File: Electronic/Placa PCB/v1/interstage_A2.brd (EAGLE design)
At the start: 82.5 x 29 mm, 22 parts, among them J1 0532611271, J2 0532611271, Q1 PMV16XNR, U2 ATMEGA328P_TQFP, Y1 16MHz

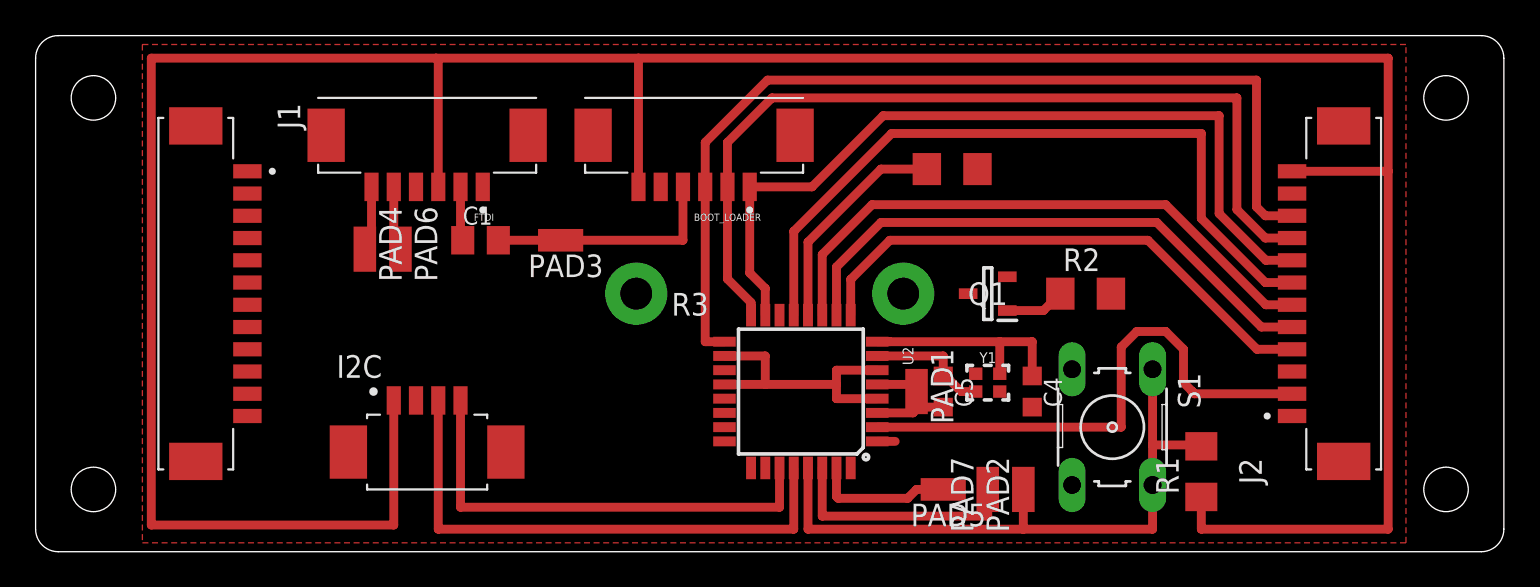
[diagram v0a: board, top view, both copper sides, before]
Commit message: Avance
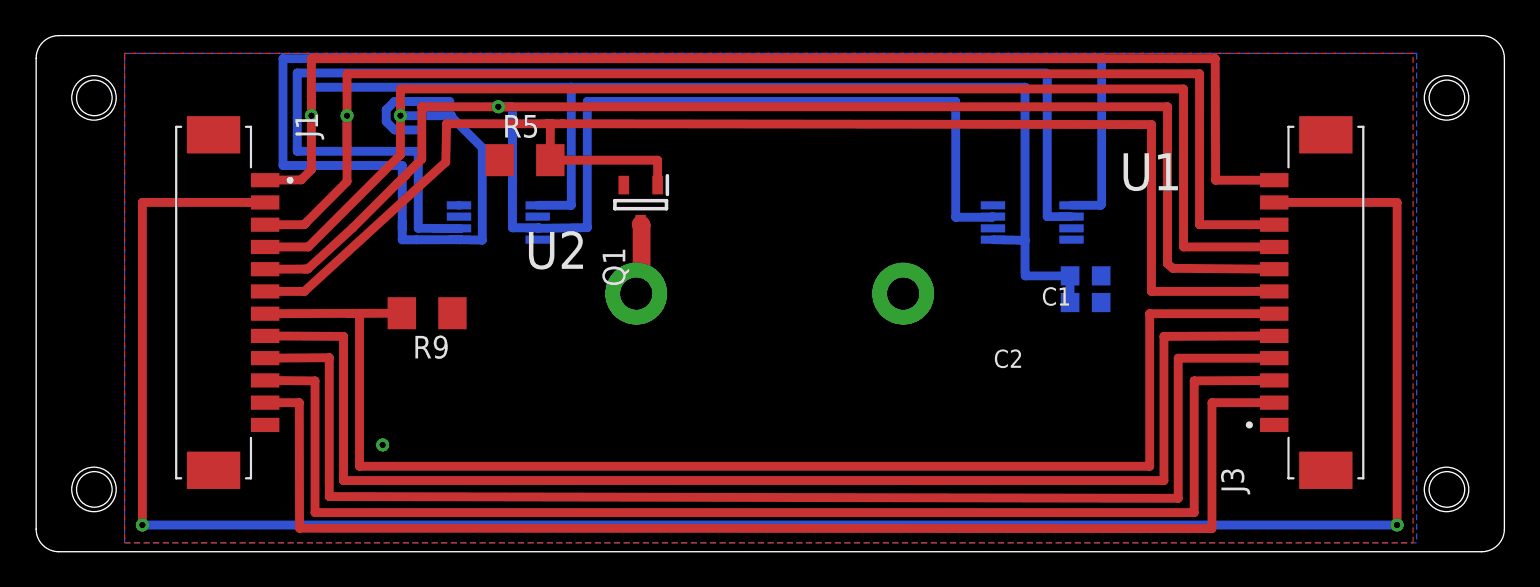
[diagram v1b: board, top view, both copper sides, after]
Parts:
- removed BOOT_LOADER, FTDI: 0532610671, picoblade6:MOLEX_0532610671
- removed C4, C5: 22pF, rcl:C0603K
- removed I2C: 0532610471, 0532610471:MOLEX_0532610471
- removed J2: 0532611271, picoblade:MOLEX_0532611271
- removed PAD1, PAD2, PAD3, PAD4, PAD5, PAD6, PAD7: WIREPADSMD1,27-254, wirepad:SMD1,27-2,54
- removed R1: 10kohm, rcl:R1206
- removed R2, R3: 330 Ohm, rcl:R1206
- removed S1: (no value), switch-omron:B3F-10XX
- removed Y1: 16MHz, SparkFun-Clocks:CRYSTAL-SMD-2.0X1.6MM
- added C2: 0.1pF, rcl:C0603K
- added J3: 0532611271, picoblade:MOLEX_0532611271
- added R5, R9: 330 Ohm, rcl:R1206
- added U1: LM70CIMM-3, LM70CIMM-3:SOP65P490X110-8N
- C1: value 100nF -> 0.1pF; device rcl:C0805K -> rcl:C0603K
- U2: value ATMEGA328P_TQFP -> LM70CIMM-3; device SparkFun-IC-Microcontroller:TQFP32-08 -> LM70CIMM-3:SOP65P490X110-8N
- moved C1 34.1 mm to (59.0, 15.5), flipped to the bottom, turned to 180 degrees
- moved Q1 20.1 mm to (34.0, 19.5), turned to 270 degrees
- moved U2 19.5 mm to (26.0, 18.5), flipped to the bottom
- moved J1 1.12 mm to (10.0, 14.0)
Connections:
- net N$4 renamed MOSFET
- removed net DTR: C1.1, FTDI.2
- removed net ICP: R3.1, U2.12
- removed net INT1: Q1.1, R2.1, U2.1
- removed net N$1: C5.1, U2.7, Y1.1
- removed net N$18: R3.2
- removed net N$2: C4.1, U2.8, Y1.3
- removed net N$6: U2.14
- removed net RST: BOOT_LOADER.4, C1.2, PAD2.1, PAD3.1, R1.2, S1.1, S1.2, U2.29
- removed net RXD: FTDI.5, PAD6.1, PAD7.1, U2.30
- removed net SCL: I2C.3, U2.28
- removed net SDA: I2C.4, U2.27
- removed net TXD: FTDI.6, PAD4.1, PAD5.1, U2.31
- new net N$3: J3.1
- new net N$4: R9.1
- net AIN0: now also J1.8, J3.5; no longer J2.5, U2.10
- net AIN1: now also J1.7, J3.6, R9.2; no longer J2.6, U2.11
- net GND: now also C1.2, C2.2, J1.2, J3.11, R5.1, U1.4, U2.4; no longer BOOT_LOADER.5, C4.2, C5.2, FTDI.4, I2C.2, J2.11, PAD1.1, R2.2, S1.3, S1.4, U2.3, U2.5
- net INT0: now also J1.10, J3.3; no longer J2.3, U2.32
- net MISO: now also J1.4, J3.9, U1.1, U2.1; no longer BOOT_LOADER.2, J2.9, U2.16
- net MOSI: now also J1.5, J3.8, U1.7, U2.7; no longer BOOT_LOADER.1, J2.8, U2.15
- net OC1A: now also J1.6, J3.7, Q1.1, R5.2; no longer J2.7, U2.13
- net SCK: now also J1.3, J3.10, U1.2, U2.2; no longer BOOT_LOADER.3, J2.10, U2.17
- net T0: now also J1.11, J3.2; no longer J2.2, U2.2
- net T1: now also J1.9, J3.4; no longer J2.4, U2.9
- net VCC: now also C1.1, C2.1, J1.1, J3.12, U1.5, U2.5; no longer BOOT_LOADER.6, FTDI.3, I2C.1, J2.12, R1.1, U2.18, U2.20, U2.4, U2.6
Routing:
- net GND: track 6.72 -> 127.8 mm, vias 0 -> 3
- net MISO: track 50.0 -> 160.2 mm, vias 0 -> 1
- net SCK: track 54.0 -> 143.5 mm, vias 0 -> 1
- net MOSI: track 46.3 -> 119.4 mm, vias 0 -> 1
- net INT0: track 0.00 -> 71.5 mm
- net VCC: track 191.4 -> 136.6 mm, vias 0 -> 1
- net RST: track 50.2 -> 0.00 mm
- net AIN1: track 33.3 -> 76.2 mm
- net T1: track 30.3 -> 72.4 mm
- net AIN0: track 32.0 -> 72.9 mm
- net T0: track 30.8 -> 70.8 mm
- net OC1A: track 41.3 -> 80.5 mm
- net SCL: track 30.6 -> 0.00 mm
- net SDA: track 26.1 -> 0.00 mm
- net RXD: track 17.2 -> 0.00 mm
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- added copper zone on layer 16, net GND
